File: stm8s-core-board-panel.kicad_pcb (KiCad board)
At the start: 2 copper layers, 95.5 x 95.5 mm, 336 parts, among them IC1 STM8S003F3P, P1 CONN_01X06, P2 USB_OTG, P3 CONN_01X09, P4 CONN_01X09, P5 CONN_01X02, SW1 SW_PUSH, U1 AS1117-5.0, Y1 16MHz

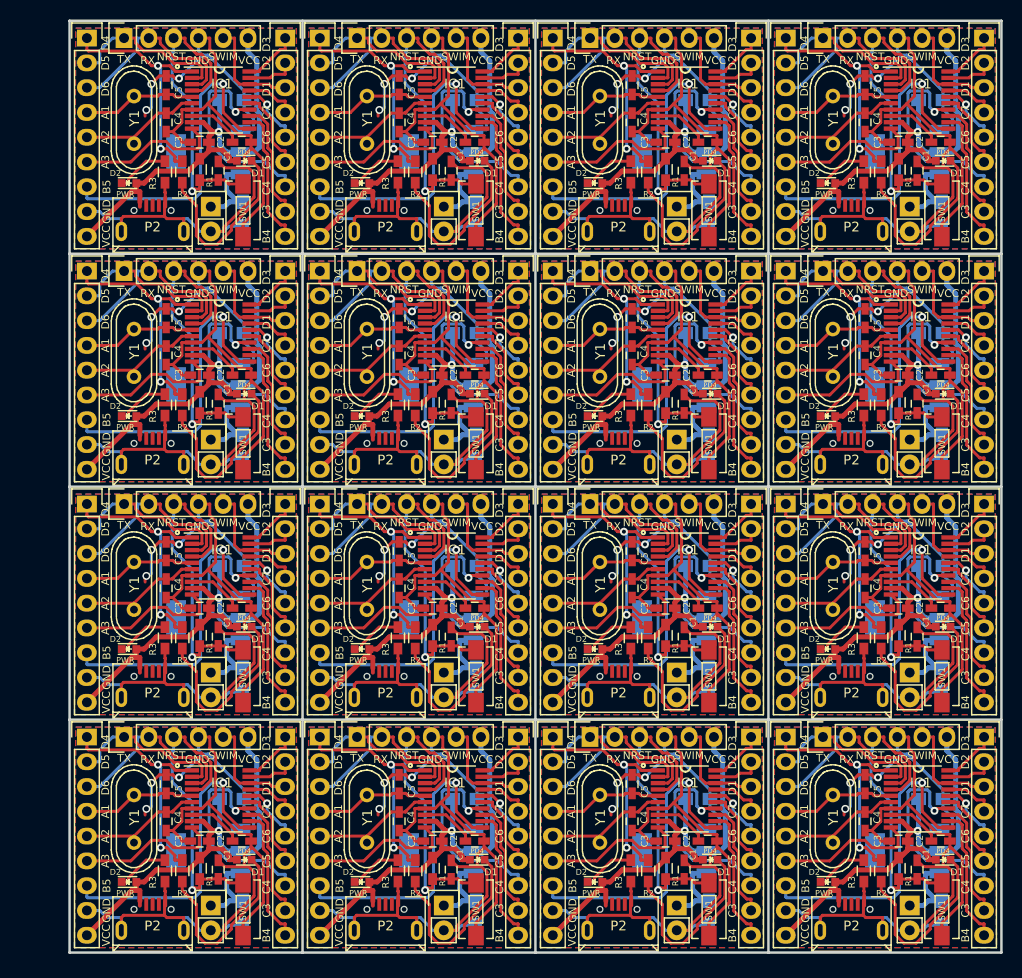
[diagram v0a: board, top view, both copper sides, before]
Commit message: forgot commit for long time. don't know what changed
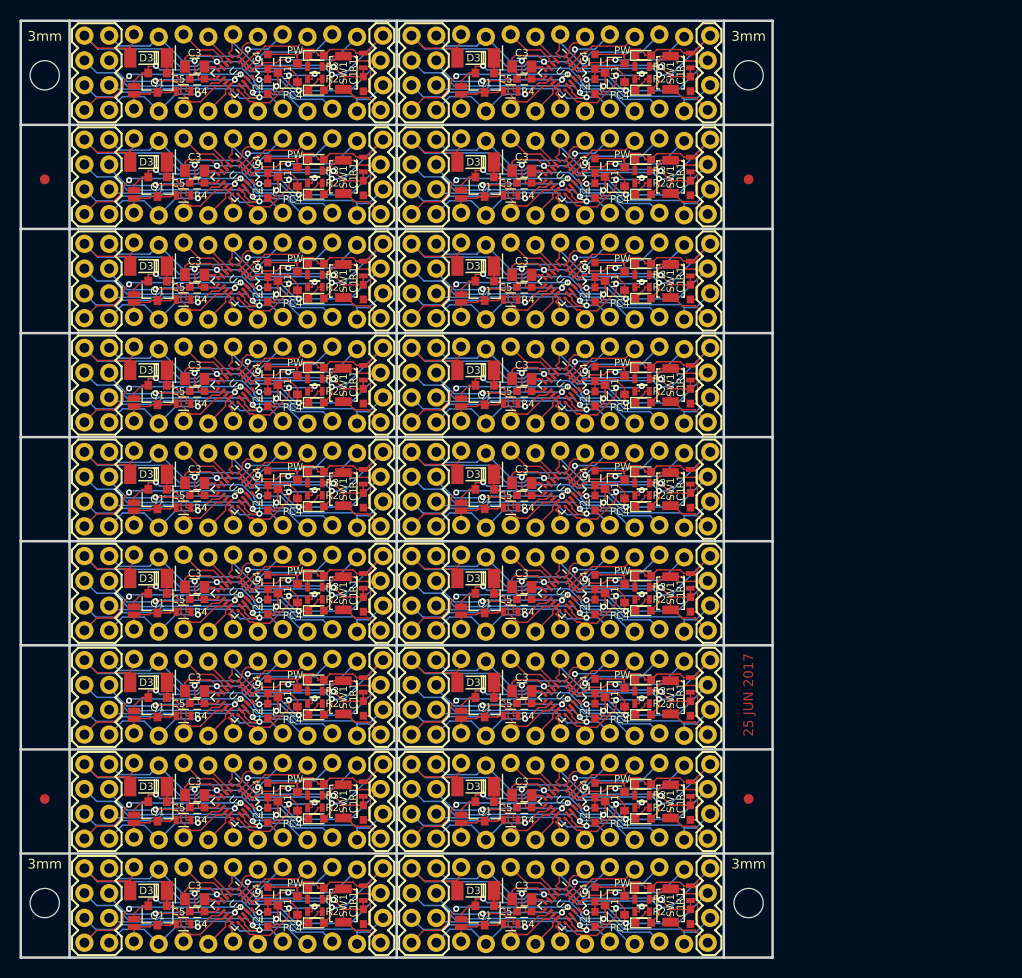
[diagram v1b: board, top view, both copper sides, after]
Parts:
- removed the C1 at (99.6, 99.7)
- removed the C1 at (51.8, 75.8)
- removed the C1 at (51.8, 51.9)
- removed the C1 at (51.8, 28.1)
- removed the C1 at (27.9, 99.7)
- removed the C1 at (27.9, 75.8)
- removed the C1 at (27.9, 51.9)
- removed the C1 at (27.9, 28.1)
- removed the C1 at (99.6, 75.8)
- removed the C1 at (99.6, 51.9)
- removed the C1 at (99.6, 28.1)
- removed the C1 at (75.7, 99.7)
- removed the C1 at (75.7, 75.8)
- removed the C1 at (75.7, 51.9)
- removed the C1 at (75.7, 28.1)
- removed the C1 at (51.8, 99.7)
- removed the C2 at (102.0, 96.8)
- removed the C2 at (54.2, 72.9)
- removed the C2 at (54.2, 49.0)
- removed the C2 at (54.2, 25.1)
- removed the C2 at (30.4, 96.8)
- removed the C2 at (30.4, 72.9)
- removed the C2 at (30.4, 49.0)
- removed the C2 at (30.4, 25.1)
- removed the C2 at (102.0, 72.9)
- removed the C2 at (102.0, 49.0)
- removed the C2 at (102.0, 25.1)
- removed the C2 at (78.1, 96.8)
- removed the C2 at (78.1, 72.9)
- removed the C2 at (78.1, 49.0)
- removed the C2 at (78.1, 25.1)
- removed the C2 at (54.2, 96.8)
- removed the C3 at (97.7, 96.8)
- removed the C3 at (49.9, 72.9)
- removed the C3 at (49.9, 49.0)
- removed the C3 at (49.9, 25.1)
- removed the C3 at (26.0, 96.8)
- removed the C3 at (26.0, 72.9)
- removed the C3 at (26.0, 49.0)
- removed the C3 at (26.0, 25.1)
- removed the C3 at (97.7, 72.9)
- removed the C3 at (97.7, 49.0)
- removed the C3 at (97.7, 25.1)
- removed the C3 at (73.8, 96.8)
- removed the C3 at (73.8, 72.9)
- removed the C3 at (73.8, 49.0)
- removed the C3 at (73.8, 25.1)
- removed the C3 at (49.9, 96.8)
- removed the C4 at (94.2, 94.7)
- removed the C4 at (46.5, 70.9)
- removed the C4 at (46.5, 47.0)
- removed the C4 at (46.5, 23.1)
- removed the C4 at (22.6, 94.7)
- removed the C4 at (22.6, 70.9)
- removed the C4 at (22.6, 47.0)
- removed the C4 at (22.6, 23.1)
- removed the C4 at (94.2, 70.9)
- removed the C4 at (94.2, 47.0)
- removed the C4 at (94.2, 23.1)
- removed the C4 at (70.4, 94.7)
- removed the C4 at (70.4, 70.9)
- removed the C4 at (70.4, 47.0)
- removed the C4 at (70.4, 23.1)
- removed the C4 at (46.5, 94.7)
- removed the C5 at (94.2, 90.9)
- removed the C5 at (46.5, 67.1)
- removed the C5 at (46.5, 43.2)
- removed the C5 at (46.5, 19.3)
- removed the C5 at (22.6, 90.9)
- removed the C5 at (22.6, 67.1)
- removed the C5 at (22.6, 43.2)
- removed the C5 at (22.6, 19.3)
- removed the C5 at (94.2, 67.1)
- removed the C5 at (94.2, 43.2)
- removed the C5 at (94.2, 19.3)
- removed the C5 at (70.4, 90.9)
- removed the C5 at (70.4, 67.1)
- removed the C5 at (70.4, 43.2)
- removed the C5 at (70.4, 19.3)
- removed the C5 at (46.5, 90.9)
- removed C6 (x16), C7 (x16): 10uF, Capacitors_SMD:C_0805_HandSoldering
- removed the D1 at (102.2, 98.7)
- removed the D1 at (54.5, 74.8)
- removed the D1 at (54.5, 50.9)
- removed the D1 at (54.5, 27.1)
- removed the D1 at (30.6, 98.7)
- removed the D1 at (30.6, 74.8)
- removed the D1 at (30.6, 50.9)
- removed the D1 at (30.6, 27.1)
- removed the D1 at (102.2, 74.8)
- removed the D1 at (102.2, 50.9)
- removed the D1 at (102.2, 27.1)
- removed the D1 at (78.4, 98.7)
- removed the D1 at (78.4, 74.8)
- removed the D1 at (78.4, 50.9)
- removed the D1 at (78.4, 27.1)
- removed the D1 at (54.5, 98.7)
- removed the D2 at (90.4, 101.0)
- removed the D2 at (42.7, 77.1)
- removed the D2 at (42.7, 53.2)
- removed the D2 at (42.7, 29.3)
- removed the D2 at (18.8, 101.0)
- removed the D2 at (18.8, 77.1)
- removed the D2 at (18.8, 53.2)
- removed the D2 at (18.8, 29.3)
- removed the D2 at (90.4, 77.1)
- removed the D2 at (90.4, 53.2)
- removed the D2 at (90.4, 29.3)
- removed the D2 at (66.5, 101.0)
- removed the D2 at (66.5, 77.1)
- removed the D2 at (66.5, 53.2)
- removed the D2 at (66.5, 29.3)
- removed the D2 at (42.7, 101.0)
- removed IC1 (x16): STM8S003F3P, Housings_SSOP:TSSOP-20_4.4x6.5mm_Pitch0.65mm
- removed P1 (x16): CONN_01X06, Pin_Headers:Pin_Header_Straight_1x06
- removed P2 (x16): USB_OTG, USB_Micro-B_MK5P
- removed P3 (x16), P4 (x16): CONN_01X09, Pin_Headers:Pin_Header_Straight_1x09
- removed P5 (x16): CONN_01X02, Pin_Headers:Pin_Header_Straight_1x02
- removed the R1 at (97.7, 99.6)
- removed the R1 at (49.9, 75.7)
- removed the R1 at (49.9, 51.8)
- removed the R1 at (49.9, 27.9)
- removed the R1 at (26.0, 99.6)
- removed the R1 at (26.0, 75.7)
- removed the R1 at (26.0, 51.8)
- removed the R1 at (26.0, 27.9)
- removed the R1 at (97.7, 75.7)
- removed the R1 at (97.7, 51.8)
- removed the R1 at (97.7, 27.9)
- removed the R1 at (73.8, 99.6)
- removed the R1 at (73.8, 75.7)
- removed the R1 at (73.8, 51.8)
- removed the R1 at (73.8, 27.9)
- removed the R1 at (49.9, 99.6)
- removed the R2 at (95.9, 99.8)
- removed the R2 at (48.1, 75.9)
- removed the R2 at (48.1, 52.1)
- removed the R2 at (48.1, 28.2)
- removed the R2 at (24.3, 99.8)
- removed the R2 at (24.3, 75.9)
- removed the R2 at (24.3, 52.1)
- removed the R2 at (24.3, 28.2)
- removed the R2 at (95.9, 75.9)
- removed the R2 at (95.9, 52.1)
- removed the R2 at (95.9, 28.2)
- removed the R2 at (72.0, 99.8)
- removed the R2 at (72.0, 75.9)
- removed the R2 at (72.0, 52.1)
- removed the R2 at (72.0, 28.2)
- removed the R2 at (48.1, 99.8)
- removed the R3 at (94.1, 99.8)
- removed the R3 at (46.4, 75.9)
- removed the R3 at (46.4, 52.1)
- removed the R3 at (46.4, 28.2)
- removed the R3 at (22.5, 99.8)
- removed the R3 at (22.5, 75.9)
- removed the R3 at (22.5, 52.1)
- removed the R3 at (22.5, 28.2)
- removed the R3 at (94.1, 75.9)
- removed the R3 at (94.1, 52.1)
- removed the R3 at (94.1, 28.2)
- removed the R3 at (70.2, 99.8)
- removed the R3 at (70.2, 75.9)
- removed the R3 at (70.2, 52.1)
- removed the R3 at (70.2, 28.2)
- removed the R3 at (46.4, 99.8)
- removed the SW1 at (102.1, 103.8)
- removed the SW1 at (54.4, 79.9)
- removed the SW1 at (54.4, 56.0)
- removed the SW1 at (54.4, 32.1)
- removed the SW1 at (30.5, 103.8)
- removed the SW1 at (30.5, 79.9)
- removed the SW1 at (30.5, 56.0)
- removed the SW1 at (30.5, 32.1)
- removed the SW1 at (102.1, 79.9)
- removed the SW1 at (102.1, 56.0)
- removed the SW1 at (102.1, 32.1)
- removed the SW1 at (78.2, 103.8)
- removed the SW1 at (78.2, 79.9)
- removed the SW1 at (78.2, 56.0)
- removed the SW1 at (78.2, 32.1)
- removed the SW1 at (54.4, 103.8)
- removed the U1 at (98.6, 97.8)
- removed the U1 at (50.8, 73.9)
- removed the U1 at (50.8, 50.0)
- removed the U1 at (50.8, 26.2)
- removed the U1 at (26.9, 97.8)
- removed the U1 at (26.9, 73.9)
- removed the U1 at (26.9, 50.0)
- removed the U1 at (26.9, 26.2)
- removed the U1 at (98.6, 73.9)
- removed the U1 at (98.6, 50.0)
- removed the U1 at (98.6, 26.2)
- removed the U1 at (74.7, 97.8)
- removed the U1 at (74.7, 73.9)
- removed the U1 at (74.7, 50.0)
- removed the U1 at (74.7, 26.2)
- removed the U1 at (50.8, 97.8)
- removed Y1 (x16): 16MHz, Crystals:Crystal_HC49-U_Vertical
- added 3mm: MountingHole_3mm, Mounting_Holes:MountingHole_3mm, F.Cu at (10.2, 103.1)
- added 3mm: MountingHole_3mm, Mounting_Holes:MountingHole_3mm, F.Cu at (82.3, 103.1)
- added 3mm: MountingHole_3mm, Mounting_Holes:MountingHole_3mm, F.Cu at (10.2, 18.3)
- added 3mm: MountingHole_3mm, Mounting_Holes:MountingHole_3mm, F.Cu at (82.3, 18.3)
- added C1: 0.1uF, Capacitors_SMD:C_0603, F.Cu at (76.3, 104.5)
- added C1: 0.1uF, Capacitors_SMD:C_0603, F.Cu at (42.8, 104.5)
- added C1: 0.1uF, Capacitors_SMD:C_0603, F.Cu at (42.8, 93.9)
- added C1: 0.1uF, Capacitors_SMD:C_0603, F.Cu at (42.8, 83.2)
- added C1: 0.1uF, Capacitors_SMD:C_0603, F.Cu at (42.8, 72.5)
- added C1: 0.1uF, Capacitors_SMD:C_0603, F.Cu at (42.8, 61.8)
- added C1: 0.1uF, Capacitors_SMD:C_0603, F.Cu at (42.8, 51.2)
- added C1: 0.1uF, Capacitors_SMD:C_0603, F.Cu at (42.8, 40.5)
- added C1: 0.1uF, Capacitors_SMD:C_0603, F.Cu at (42.8, 29.8)
- added C1: 0.1uF, Capacitors_SMD:C_0603, F.Cu at (42.8, 19.2)
- added C1: 0.1uF, Capacitors_SMD:C_0603, F.Cu at (76.3, 93.9)
- added C1: 0.1uF, Capacitors_SMD:C_0603, F.Cu at (76.3, 83.2)
- added C1: 0.1uF, Capacitors_SMD:C_0603, F.Cu at (76.3, 72.5)
- added C1: 0.1uF, Capacitors_SMD:C_0603, F.Cu at (76.3, 61.8)
- added C1: 0.1uF, Capacitors_SMD:C_0603, F.Cu at (76.3, 51.2)
- added C1: 0.1uF, Capacitors_SMD:C_0603, F.Cu at (76.3, 40.5)
- added C1: 0.1uF, Capacitors_SMD:C_0603, F.Cu at (76.3, 29.8)
- added C1: 0.1uF, Capacitors_SMD:C_0603, F.Cu at (76.3, 19.2)
- added C2: 1uF, Capacitors_SMD:C_0603, F.Cu at (66.5, 104.8)
- added C2: 1uF, Capacitors_SMD:C_0603, F.Cu at (33.0, 104.8)
- added C2: 1uF, Capacitors_SMD:C_0603, F.Cu at (33.0, 94.1)
- added C2: 1uF, Capacitors_SMD:C_0603, F.Cu at (33.0, 83.4)
- added C2: 1uF, Capacitors_SMD:C_0603, F.Cu at (33.0, 72.8)
- added C2: 1uF, Capacitors_SMD:C_0603, F.Cu at (33.0, 62.1)
- added C2: 1uF, Capacitors_SMD:C_0603, F.Cu at (33.0, 51.4)
- added C2: 1uF, Capacitors_SMD:C_0603, F.Cu at (33.0, 40.8)
- added C2: 1uF, Capacitors_SMD:C_0603, F.Cu at (33.0, 30.1)
- added C2: 1uF, Capacitors_SMD:C_0603, F.Cu at (33.0, 19.4)
- added C2: 1uF, Capacitors_SMD:C_0603, F.Cu at (66.5, 94.1)
- added C2: 1uF, Capacitors_SMD:C_0603, F.Cu at (66.5, 83.4)
- added C2: 1uF, Capacitors_SMD:C_0603, F.Cu at (66.5, 72.8)
- added C2: 1uF, Capacitors_SMD:C_0603, F.Cu at (66.5, 62.1)
- added C2: 1uF, Capacitors_SMD:C_0603, F.Cu at (66.5, 51.4)
- added C2: 1uF, Capacitors_SMD:C_0603, F.Cu at (66.5, 40.8)
- added C2: 1uF, Capacitors_SMD:C_0603, F.Cu at (66.5, 30.1)
- added C2: 1uF, Capacitors_SMD:C_0603, F.Cu at (66.5, 19.4)
- added C3: 1.0uF, Capacitors_SMD:C_0805, F.Cu at (59.1, 102.7)
- added C3: 1.0uF, Capacitors_SMD:C_0805, F.Cu at (25.5, 102.7)
- added C3: 1.0uF, Capacitors_SMD:C_0805, F.Cu at (25.5, 92.1)
- added C3: 1.0uF, Capacitors_SMD:C_0805, F.Cu at (25.5, 81.4)
- added C3: 1.0uF, Capacitors_SMD:C_0805, F.Cu at (25.5, 70.7)
- added C3: 1.0uF, Capacitors_SMD:C_0805, F.Cu at (25.5, 60.1)
- added C3: 1.0uF, Capacitors_SMD:C_0805, F.Cu at (25.5, 49.4)
- added C3: 1.0uF, Capacitors_SMD:C_0805, F.Cu at (25.5, 38.7)
- added C3: 1.0uF, Capacitors_SMD:C_0805, F.Cu at (25.5, 28.1)
- added C3: 1.0uF, Capacitors_SMD:C_0805, F.Cu at (25.5, 17.4)
- added C3: 1.0uF, Capacitors_SMD:C_0805, F.Cu at (59.1, 92.1)
- added C3: 1.0uF, Capacitors_SMD:C_0805, F.Cu at (59.1, 81.4)
- added C3: 1.0uF, Capacitors_SMD:C_0805, F.Cu at (59.1, 70.7)
- added C3: 1.0uF, Capacitors_SMD:C_0805, F.Cu at (59.1, 60.1)
- added C3: 1.0uF, Capacitors_SMD:C_0805, F.Cu at (59.1, 49.4)
- added C3: 1.0uF, Capacitors_SMD:C_0805, F.Cu at (59.1, 38.7)
- added C3: 1.0uF, Capacitors_SMD:C_0805, F.Cu at (59.1, 28.1)
- added C3: 1.0uF, Capacitors_SMD:C_0805, F.Cu at (59.1, 17.4)
- added C4: 1uF, Capacitors_SMD:C_0603, F.Cu at (66.5, 102.2)
- added C4: 1uF, Capacitors_SMD:C_0603, F.Cu at (33.0, 102.2)
- added C4: 1uF, Capacitors_SMD:C_0603, F.Cu at (33.0, 91.6)
- added C4: 1uF, Capacitors_SMD:C_0603, F.Cu at (33.0, 80.9)
- added C4: 1uF, Capacitors_SMD:C_0603, F.Cu at (33.0, 70.2)
- added C4: 1uF, Capacitors_SMD:C_0603, F.Cu at (33.0, 59.6)
- added C4: 1uF, Capacitors_SMD:C_0603, F.Cu at (33.0, 48.9)
- added C4: 1uF, Capacitors_SMD:C_0603, F.Cu at (33.0, 38.2)
- added C4: 1uF, Capacitors_SMD:C_0603, F.Cu at (33.0, 27.6)
- added C4: 1uF, Capacitors_SMD:C_0603, F.Cu at (33.0, 16.9)
- added C4: 1uF, Capacitors_SMD:C_0603, F.Cu at (66.5, 91.6)
- added C4: 1uF, Capacitors_SMD:C_0603, F.Cu at (66.5, 80.9)
- added C4: 1uF, Capacitors_SMD:C_0603, F.Cu at (66.5, 70.2)
- added C4: 1uF, Capacitors_SMD:C_0603, F.Cu at (66.5, 59.6)
- added C4: 1uF, Capacitors_SMD:C_0603, F.Cu at (66.5, 48.9)
- added C4: 1uF, Capacitors_SMD:C_0603, F.Cu at (66.5, 38.2)
- added C4: 1uF, Capacitors_SMD:C_0603, F.Cu at (66.5, 27.6)
- added C4: 1uF, Capacitors_SMD:C_0603, F.Cu at (66.5, 16.9)
- added C5: 0.1uF, Capacitors_SMD:C_0603, F.Cu at (59.3, 104.0)
- added C5: 0.1uF, Capacitors_SMD:C_0603, F.Cu at (25.8, 104.0)
- added C5: 0.1uF, Capacitors_SMD:C_0603, F.Cu at (25.8, 93.3)
- added C5: 0.1uF, Capacitors_SMD:C_0603, F.Cu at (25.8, 82.7)
- added C5: 0.1uF, Capacitors_SMD:C_0603, F.Cu at (25.8, 72.0)
- added C5: 0.1uF, Capacitors_SMD:C_0603, F.Cu at (25.8, 61.3)
- added C5: 0.1uF, Capacitors_SMD:C_0603, F.Cu at (25.8, 50.7)
- added C5: 0.1uF, Capacitors_SMD:C_0603, F.Cu at (25.8, 40.0)
- added C5: 0.1uF, Capacitors_SMD:C_0603, F.Cu at (25.8, 29.3)
- added C5: 0.1uF, Capacitors_SMD:C_0603, F.Cu at (25.8, 18.7)
- added C5: 0.1uF, Capacitors_SMD:C_0603, F.Cu at (59.3, 93.3)
- added C5: 0.1uF, Capacitors_SMD:C_0603, F.Cu at (59.3, 82.7)
- added C5: 0.1uF, Capacitors_SMD:C_0603, F.Cu at (59.3, 72.0)
- added C5: 0.1uF, Capacitors_SMD:C_0603, F.Cu at (59.3, 61.3)
- added C5: 0.1uF, Capacitors_SMD:C_0603, F.Cu at (59.3, 50.7)
- added C5: 0.1uF, Capacitors_SMD:C_0603, F.Cu at (59.3, 40.0)
- added C5: 0.1uF, Capacitors_SMD:C_0603, F.Cu at (59.3, 29.3)
- added C5: 0.1uF, Capacitors_SMD:C_0603, F.Cu at (59.3, 18.7)
- added D1: BLUE, LEDs:LED_0603, F.Cu at (71.5, 105.2)
- added D1: BLUE, LEDs:LED_0603, F.Cu at (38.0, 105.2)
- added D1: BLUE, LEDs:LED_0603, F.Cu at (38.0, 94.5)
- added D1: BLUE, LEDs:LED_0603, F.Cu at (38.0, 83.8)
- added D1: BLUE, LEDs:LED_0603, F.Cu at (38.0, 73.2)
- added D1: BLUE, LEDs:LED_0603, F.Cu at (38.0, 62.5)
- added D1: BLUE, LEDs:LED_0603, F.Cu at (38.0, 51.8)
- added D1: BLUE, LEDs:LED_0603, F.Cu at (38.0, 41.1)
- added D1: BLUE, LEDs:LED_0603, F.Cu at (38.0, 30.5)
- added D1: BLUE, LEDs:LED_0603, F.Cu at (38.0, 19.8)
- added D1: BLUE, LEDs:LED_0603, F.Cu at (71.5, 94.5)
- added D1: BLUE, LEDs:LED_0603, F.Cu at (71.5, 83.8)
- added D1: BLUE, LEDs:LED_0603, F.Cu at (71.5, 73.2)
- added D1: BLUE, LEDs:LED_0603, F.Cu at (71.5, 62.5)
- added D1: BLUE, LEDs:LED_0603, F.Cu at (71.5, 51.8)
- added D1: BLUE, LEDs:LED_0603, F.Cu at (71.5, 41.1)
- added D1: BLUE, LEDs:LED_0603, F.Cu at (71.5, 30.5)
- added D1: BLUE, LEDs:LED_0603, F.Cu at (71.5, 19.8)
- added D2: RED, LEDs:LED_0603, F.Cu at (71.5, 101.6)
- added D2: RED, LEDs:LED_0603, F.Cu at (38.0, 101.6)
- added D2: RED, LEDs:LED_0603, F.Cu at (38.0, 90.9)
- added D2: RED, LEDs:LED_0603, F.Cu at (38.0, 80.3)
- added D2: RED, LEDs:LED_0603, F.Cu at (38.0, 69.6)
- added D2: RED, LEDs:LED_0603, F.Cu at (38.0, 58.9)
- added D2: RED, LEDs:LED_0603, F.Cu at (38.0, 48.3)
- added D2: RED, LEDs:LED_0603, F.Cu at (38.0, 37.6)
- added D2: RED, LEDs:LED_0603, F.Cu at (38.0, 26.9)
- added D2: RED, LEDs:LED_0603, F.Cu at (38.0, 16.3)
- added D2: RED, LEDs:LED_0603, F.Cu at (71.5, 90.9)
- added D2: RED, LEDs:LED_0603, F.Cu at (71.5, 80.3)
- added D2: RED, LEDs:LED_0603, F.Cu at (71.5, 69.6)
- added D2: RED, LEDs:LED_0603, F.Cu at (71.5, 58.9)
- added D2: RED, LEDs:LED_0603, F.Cu at (71.5, 48.3)
- added D2: RED, LEDs:LED_0603, F.Cu at (71.5, 37.6)
- added D2: RED, LEDs:LED_0603, F.Cu at (71.5, 26.9)
- added D2: RED, LEDs:LED_0603, F.Cu at (71.5, 16.3)
- added D3: 5.6V, MyOwn:SOD-80, F.Cu at (54.3, 101.9)
- added D3: 5.6V, MyOwn:SOD-80, F.Cu at (20.8, 101.9)
- added D3: 5.6V, MyOwn:SOD-80, F.Cu at (20.8, 91.2)
- added D3: 5.6V, MyOwn:SOD-80, F.Cu at (20.8, 80.5)
- added D3: 5.6V, MyOwn:SOD-80, F.Cu at (20.8, 69.8)
- added D3: 5.6V, MyOwn:SOD-80, F.Cu at (20.8, 59.2)
- added D3: 5.6V, MyOwn:SOD-80, F.Cu at (20.8, 48.5)
- added D3: 5.6V, MyOwn:SOD-80, F.Cu at (20.8, 37.8)
- added D3: 5.6V, MyOwn:SOD-80, F.Cu at (20.8, 27.2)
- added D3: 5.6V, MyOwn:SOD-80, F.Cu at (20.8, 16.5)
- added D3: 5.6V, MyOwn:SOD-80, F.Cu at (54.3, 91.2)
- added D3: 5.6V, MyOwn:SOD-80, F.Cu at (54.3, 80.5)
- added D3: 5.6V, MyOwn:SOD-80, F.Cu at (54.3, 69.8)
- added D3: 5.6V, MyOwn:SOD-80, F.Cu at (54.3, 59.2)
- added D3: 5.6V, MyOwn:SOD-80, F.Cu at (54.3, 48.5)
- added D3: 5.6V, MyOwn:SOD-80, F.Cu at (54.3, 37.8)
- added D3: 5.6V, MyOwn:SOD-80, F.Cu at (54.3, 27.2)
- added D3: 5.6V, MyOwn:SOD-80, F.Cu at (54.3, 16.5)
- added J1: CONN_01X04, SparkFun-Connectors:1X04_LOCK, F.Cu at (78.2, 107.2)
- added J1: CONN_01X04, SparkFun-Connectors:1X04_LOCK, F.Cu at (44.7, 107.2)
- added J1: CONN_01X04, SparkFun-Connectors:1X04_LOCK, F.Cu at (44.7, 96.5)
- added J1: CONN_01X04, SparkFun-Connectors:1X04_LOCK, F.Cu at (44.7, 85.9)
- added J1: CONN_01X04, SparkFun-Connectors:1X04_LOCK, F.Cu at (44.7, 75.2)
- added J1: CONN_01X04, SparkFun-Connectors:1X04_LOCK, F.Cu at (44.7, 64.5)
- added J1: CONN_01X04, SparkFun-Connectors:1X04_LOCK, F.Cu at (44.7, 53.8)
- added J1: CONN_01X04, SparkFun-Connectors:1X04_LOCK, F.Cu at (44.7, 43.2)
- added J1: CONN_01X04, SparkFun-Connectors:1X04_LOCK, F.Cu at (44.7, 32.5)
- added J1: CONN_01X04, SparkFun-Connectors:1X04_LOCK, F.Cu at (44.7, 21.8)
- added J1: CONN_01X04, SparkFun-Connectors:1X04_LOCK, F.Cu at (78.2, 96.5)
- added J1: CONN_01X04, SparkFun-Connectors:1X04_LOCK, F.Cu at (78.2, 85.9)
- added J1: CONN_01X04, SparkFun-Connectors:1X04_LOCK, F.Cu at (78.2, 75.2)
- added J1: CONN_01X04, SparkFun-Connectors:1X04_LOCK, F.Cu at (78.2, 64.5)
- added J1: CONN_01X04, SparkFun-Connectors:1X04_LOCK, F.Cu at (78.2, 53.8)
- added J1: CONN_01X04, SparkFun-Connectors:1X04_LOCK, F.Cu at (78.2, 43.2)
- added J1: CONN_01X04, SparkFun-Connectors:1X04_LOCK, F.Cu at (78.2, 32.5)
- added J1: CONN_01X04, SparkFun-Connectors:1X04_LOCK, F.Cu at (78.2, 21.8)
- added J2: CONN_02X04, SparkFun-Connectors:2X4, F.Cu at (49.0, 103.4)
- added J2: CONN_02X04, SparkFun-Connectors:2X4, F.Cu at (15.5, 103.4)
- added J2: CONN_02X04, SparkFun-Connectors:2X4, F.Cu at (15.5, 92.7)
- added J2: CONN_02X04, SparkFun-Connectors:2X4, F.Cu at (15.5, 82.0)
- added J2: CONN_02X04, SparkFun-Connectors:2X4, F.Cu at (15.5, 71.4)
- added J2: CONN_02X04, SparkFun-Connectors:2X4, F.Cu at (15.5, 60.7)
- added J2: CONN_02X04, SparkFun-Connectors:2X4, F.Cu at (15.5, 50.0)
- added J2: CONN_02X04, SparkFun-Connectors:2X4, F.Cu at (15.5, 39.4)
- added J2: CONN_02X04, SparkFun-Connectors:2X4, F.Cu at (15.5, 28.7)
- added J2: CONN_02X04, SparkFun-Connectors:2X4, F.Cu at (15.5, 18.0)
- added J2: CONN_02X04, SparkFun-Connectors:2X4, F.Cu at (49.0, 92.7)
- added J2: CONN_02X04, SparkFun-Connectors:2X4, F.Cu at (49.0, 82.0)
- added J2: CONN_02X04, SparkFun-Connectors:2X4, F.Cu at (49.0, 71.4)
- added J2: CONN_02X04, SparkFun-Connectors:2X4, F.Cu at (49.0, 60.7)
- added J2: CONN_02X04, SparkFun-Connectors:2X4, F.Cu at (49.0, 50.0)
- added J2: CONN_02X04, SparkFun-Connectors:2X4, F.Cu at (49.0, 39.4)
- added J2: CONN_02X04, SparkFun-Connectors:2X4, F.Cu at (49.0, 28.7)
- added J2: CONN_02X04, SparkFun-Connectors:2X4, F.Cu at (49.0, 18.0)
- added J3: CONN_01X10, SparkFun-Connectors:1X10_LOCK_NS, F.Cu at (52.8, 107.2)
- added J3: CONN_01X10, SparkFun-Connectors:1X10_LOCK_NS, F.Cu at (19.3, 107.2)
- added J3: CONN_01X10, SparkFun-Connectors:1X10_LOCK_NS, F.Cu at (19.3, 96.5)
- added J3: CONN_01X10, SparkFun-Connectors:1X10_LOCK_NS, F.Cu at (19.3, 85.9)
- added J3: CONN_01X10, SparkFun-Connectors:1X10_LOCK_NS, F.Cu at (19.3, 75.2)
- added J3: CONN_01X10, SparkFun-Connectors:1X10_LOCK_NS, F.Cu at (19.3, 64.5)
- added J3: CONN_01X10, SparkFun-Connectors:1X10_LOCK_NS, F.Cu at (19.3, 53.8)
- added J3: CONN_01X10, SparkFun-Connectors:1X10_LOCK_NS, F.Cu at (19.3, 43.2)
- added J3: CONN_01X10, SparkFun-Connectors:1X10_LOCK_NS, F.Cu at (19.3, 32.5)
- added J3: CONN_01X10, SparkFun-Connectors:1X10_LOCK_NS, F.Cu at (19.3, 21.8)
- added J3: CONN_01X10, SparkFun-Connectors:1X10_LOCK_NS, F.Cu at (52.8, 96.5)
- added J3: CONN_01X10, SparkFun-Connectors:1X10_LOCK_NS, F.Cu at (52.8, 85.9)
- added J3: CONN_01X10, SparkFun-Connectors:1X10_LOCK_NS, F.Cu at (52.8, 75.2)
- added J3: CONN_01X10, SparkFun-Connectors:1X10_LOCK_NS, F.Cu at (52.8, 64.5)
- added J3: CONN_01X10, SparkFun-Connectors:1X10_LOCK_NS, F.Cu at (52.8, 53.8)
- added J3: CONN_01X10, SparkFun-Connectors:1X10_LOCK_NS, F.Cu at (52.8, 43.2)
- added J3: CONN_01X10, SparkFun-Connectors:1X10_LOCK_NS, F.Cu at (52.8, 32.5)
- added J3: CONN_01X10, SparkFun-Connectors:1X10_LOCK_NS, F.Cu at (52.8, 21.8)
- added J4: CONN_01X10, SparkFun-Connectors:1X10_LOCK_NS, F.Cu at (52.8, 99.6)
- added J4: CONN_01X10, SparkFun-Connectors:1X10_LOCK_NS, F.Cu at (19.3, 99.6)
- added J4: CONN_01X10, SparkFun-Connectors:1X10_LOCK_NS, F.Cu at (19.3, 88.9)
- added J4: CONN_01X10, SparkFun-Connectors:1X10_LOCK_NS, F.Cu at (19.3, 78.2)
- added J4: CONN_01X10, SparkFun-Connectors:1X10_LOCK_NS, F.Cu at (19.3, 67.6)
- added J4: CONN_01X10, SparkFun-Connectors:1X10_LOCK_NS, F.Cu at (19.3, 56.9)
- added J4: CONN_01X10, SparkFun-Connectors:1X10_LOCK_NS, F.Cu at (19.3, 46.2)
- added J4: CONN_01X10, SparkFun-Connectors:1X10_LOCK_NS, F.Cu at (19.3, 35.6)
- added J4: CONN_01X10, SparkFun-Connectors:1X10_LOCK_NS, F.Cu at (19.3, 24.9)
- added J4: CONN_01X10, SparkFun-Connectors:1X10_LOCK_NS, F.Cu at (19.3, 14.2)
- added J4: CONN_01X10, SparkFun-Connectors:1X10_LOCK_NS, F.Cu at (52.8, 88.9)
- added J4: CONN_01X10, SparkFun-Connectors:1X10_LOCK_NS, F.Cu at (52.8, 78.2)
- added J4: CONN_01X10, SparkFun-Connectors:1X10_LOCK_NS, F.Cu at (52.8, 67.6)
- added J4: CONN_01X10, SparkFun-Connectors:1X10_LOCK_NS, F.Cu at (52.8, 56.9)
- added J4: CONN_01X10, SparkFun-Connectors:1X10_LOCK_NS, F.Cu at (52.8, 46.2)
- added J4: CONN_01X10, SparkFun-Connectors:1X10_LOCK_NS, F.Cu at (52.8, 35.6)
- added J4: CONN_01X10, SparkFun-Connectors:1X10_LOCK_NS, F.Cu at (52.8, 24.9)
- added J4: CONN_01X10, SparkFun-Connectors:1X10_LOCK_NS, F.Cu at (52.8, 14.2)
- added JP2: 12V-30V input, SparkFun-Jumpers:SMT-JUMPER_2_NO_NO-SILK, F.Cu at (52.8, 105.2)
- added JP2: 12V-30V input, SparkFun-Jumpers:SMT-JUMPER_2_NO_NO-SILK, F.Cu at (19.3, 105.2)
- added JP2: 12V-30V input, SparkFun-Jumpers:SMT-JUMPER_2_NO_NO-SILK, F.Cu at (19.3, 94.5)
- added JP2: 12V-30V input, SparkFun-Jumpers:SMT-JUMPER_2_NO_NO-SILK, F.Cu at (19.3, 83.8)
- added JP2: 12V-30V input, SparkFun-Jumpers:SMT-JUMPER_2_NO_NO-SILK, F.Cu at (19.3, 73.2)
- added JP2: 12V-30V input, SparkFun-Jumpers:SMT-JUMPER_2_NO_NO-SILK, F.Cu at (19.3, 62.5)
- added JP2: 12V-30V input, SparkFun-Jumpers:SMT-JUMPER_2_NO_NO-SILK, F.Cu at (19.3, 51.8)
- added JP2: 12V-30V input, SparkFun-Jumpers:SMT-JUMPER_2_NO_NO-SILK, F.Cu at (19.3, 41.1)
- added JP2: 12V-30V input, SparkFun-Jumpers:SMT-JUMPER_2_NO_NO-SILK, F.Cu at (19.3, 30.5)
- added JP2: 12V-30V input, SparkFun-Jumpers:SMT-JUMPER_2_NO_NO-SILK, F.Cu at (19.3, 19.8)
- added JP2: 12V-30V input, SparkFun-Jumpers:SMT-JUMPER_2_NO_NO-SILK, F.Cu at (52.8, 94.5)
- added JP2: 12V-30V input, SparkFun-Jumpers:SMT-JUMPER_2_NO_NO-SILK, F.Cu at (52.8, 83.8)
- added JP2: 12V-30V input, SparkFun-Jumpers:SMT-JUMPER_2_NO_NO-SILK, F.Cu at (52.8, 73.2)
- added JP2: 12V-30V input, SparkFun-Jumpers:SMT-JUMPER_2_NO_NO-SILK, F.Cu at (52.8, 62.5)
- added JP2: 12V-30V input, SparkFun-Jumpers:SMT-JUMPER_2_NO_NO-SILK, F.Cu at (52.8, 51.8)
- added JP2: 12V-30V input, SparkFun-Jumpers:SMT-JUMPER_2_NO_NO-SILK, F.Cu at (52.8, 41.1)
- added JP2: 12V-30V input, SparkFun-Jumpers:SMT-JUMPER_2_NO_NO-SILK, F.Cu at (52.8, 30.5)
- added JP2: 12V-30V input, SparkFun-Jumpers:SMT-JUMPER_2_NO_NO-SILK, F.Cu at (52.8, 19.8)
- added Q1: BC817-40, TO_SOT_Packages_SMD:SOT-23, F.Cu at (55.2, 104.4)
- added Q1: BC817-40, TO_SOT_Packages_SMD:SOT-23, F.Cu at (21.7, 104.4)
- added Q1: BC817-40, TO_SOT_Packages_SMD:SOT-23, F.Cu at (21.7, 93.7)
- added Q1: BC817-40, TO_SOT_Packages_SMD:SOT-23, F.Cu at (21.7, 83.1)
- added Q1: BC817-40, TO_SOT_Packages_SMD:SOT-23, F.Cu at (21.7, 72.4)
- added Q1: BC817-40, TO_SOT_Packages_SMD:SOT-23, F.Cu at (21.7, 61.7)
- added Q1: BC817-40, TO_SOT_Packages_SMD:SOT-23, F.Cu at (21.7, 51.1)
- added Q1: BC817-40, TO_SOT_Packages_SMD:SOT-23, F.Cu at (21.7, 40.4)
- added Q1: BC817-40, TO_SOT_Packages_SMD:SOT-23, F.Cu at (21.7, 29.7)
- added Q1: BC817-40, TO_SOT_Packages_SMD:SOT-23, F.Cu at (21.7, 19.1)
- added Q1: BC817-40, TO_SOT_Packages_SMD:SOT-23, F.Cu at (55.2, 93.7)
- added Q1: BC817-40, TO_SOT_Packages_SMD:SOT-23, F.Cu at (55.2, 83.1)
- added Q1: BC817-40, TO_SOT_Packages_SMD:SOT-23, F.Cu at (55.2, 72.4)
- added Q1: BC817-40, TO_SOT_Packages_SMD:SOT-23, F.Cu at (55.2, 61.7)
- added Q1: BC817-40, TO_SOT_Packages_SMD:SOT-23, F.Cu at (55.2, 51.1)
- added Q1: BC817-40, TO_SOT_Packages_SMD:SOT-23, F.Cu at (55.2, 40.4)
- added Q1: BC817-40, TO_SOT_Packages_SMD:SOT-23, F.Cu at (55.2, 29.7)
- added Q1: BC817-40, TO_SOT_Packages_SMD:SOT-23, F.Cu at (55.2, 19.1)
- added R1: 100K, Resistors_SMD:R_0603, F.Cu at (76.3, 102.1)
- added R1: 100K, Resistors_SMD:R_0603, F.Cu at (42.8, 102.1)
- added R1: 100K, Resistors_SMD:R_0603, F.Cu at (42.8, 91.4)
- added R1: 100K, Resistors_SMD:R_0603, F.Cu at (42.8, 80.8)
- added R1: 100K, Resistors_SMD:R_0603, F.Cu at (42.8, 70.1)
- added R1: 100K, Resistors_SMD:R_0603, F.Cu at (42.8, 59.4)
- added R1: 100K, Resistors_SMD:R_0603, F.Cu at (42.8, 48.8)
- added R1: 100K, Resistors_SMD:R_0603, F.Cu at (42.8, 38.1)
- added R1: 100K, Resistors_SMD:R_0603, F.Cu at (42.8, 27.4)
- added R1: 100K, Resistors_SMD:R_0603, F.Cu at (42.8, 16.8)
- added R1: 100K, Resistors_SMD:R_0603, F.Cu at (76.3, 91.4)
- added R1: 100K, Resistors_SMD:R_0603, F.Cu at (76.3, 80.8)
- added R1: 100K, Resistors_SMD:R_0603, F.Cu at (76.3, 70.1)
- added R1: 100K, Resistors_SMD:R_0603, F.Cu at (76.3, 59.4)
- added R1: 100K, Resistors_SMD:R_0603, F.Cu at (76.3, 48.8)
- added R1: 100K, Resistors_SMD:R_0603, F.Cu at (76.3, 38.1)
- added R1: 100K, Resistors_SMD:R_0603, F.Cu at (76.3, 27.4)
- added R1: 100K, Resistors_SMD:R_0603, F.Cu at (76.3, 16.8)
- added R2: 1K, Resistors_SMD:R_0603, F.Cu at (71.4, 104.0)
- added R2: 1K, Resistors_SMD:R_0603, F.Cu at (37.8, 104.0)
- added R2: 1K, Resistors_SMD:R_0603, F.Cu at (37.8, 93.3)
- added R2: 1K, Resistors_SMD:R_0603, F.Cu at (37.8, 82.7)
- added R2: 1K, Resistors_SMD:R_0603, F.Cu at (37.8, 72.0)
- added R2: 1K, Resistors_SMD:R_0603, F.Cu at (37.8, 61.3)
- added R2: 1K, Resistors_SMD:R_0603, F.Cu at (37.8, 50.7)
- added R2: 1K, Resistors_SMD:R_0603, F.Cu at (37.8, 40.0)
- added R2: 1K, Resistors_SMD:R_0603, F.Cu at (37.8, 29.3)
- added R2: 1K, Resistors_SMD:R_0603, F.Cu at (37.8, 18.7)
- added R2: 1K, Resistors_SMD:R_0603, F.Cu at (71.4, 93.3)
- added R2: 1K, Resistors_SMD:R_0603, F.Cu at (71.4, 82.7)
- added R2: 1K, Resistors_SMD:R_0603, F.Cu at (71.4, 72.0)
- added R2: 1K, Resistors_SMD:R_0603, F.Cu at (71.4, 61.3)
- added R2: 1K, Resistors_SMD:R_0603, F.Cu at (71.4, 50.7)
- added R2: 1K, Resistors_SMD:R_0603, F.Cu at (71.4, 40.0)
- added R2: 1K, Resistors_SMD:R_0603, F.Cu at (71.4, 29.3)
- added R2: 1K, Resistors_SMD:R_0603, F.Cu at (71.4, 18.7)
- added R3: 1K, Resistors_SMD:R_0603, F.Cu at (71.4, 102.7)
- added R3: 1K, Resistors_SMD:R_0603, F.Cu at (37.8, 102.7)
- added R3: 1K, Resistors_SMD:R_0603, F.Cu at (37.8, 92.1)
- added R3: 1K, Resistors_SMD:R_0603, F.Cu at (37.8, 81.4)
- added R3: 1K, Resistors_SMD:R_0603, F.Cu at (37.8, 70.7)
- added R3: 1K, Resistors_SMD:R_0603, F.Cu at (37.8, 60.1)
- added R3: 1K, Resistors_SMD:R_0603, F.Cu at (37.8, 49.4)
- added R3: 1K, Resistors_SMD:R_0603, F.Cu at (37.8, 38.7)
- added R3: 1K, Resistors_SMD:R_0603, F.Cu at (37.8, 28.1)
- added R3: 1K, Resistors_SMD:R_0603, F.Cu at (37.8, 17.4)
- added R3: 1K, Resistors_SMD:R_0603, F.Cu at (71.4, 92.1)
- added R3: 1K, Resistors_SMD:R_0603, F.Cu at (71.4, 81.4)
- added R3: 1K, Resistors_SMD:R_0603, F.Cu at (71.4, 70.7)
- added R3: 1K, Resistors_SMD:R_0603, F.Cu at (71.4, 60.1)
- added R3: 1K, Resistors_SMD:R_0603, F.Cu at (71.4, 49.4)
- added R3: 1K, Resistors_SMD:R_0603, F.Cu at (71.4, 38.7)
- added R3: 1K, Resistors_SMD:R_0603, F.Cu at (71.4, 28.1)
- added R3: 1K, Resistors_SMD:R_0603, F.Cu at (71.4, 17.4)
- added R4: 1K, Resistors_SMD:R_0603, F.Cu at (57.9, 105.3)
- added R4: 1K, Resistors_SMD:R_0603, F.Cu at (24.4, 105.3)
- added R4: 1K, Resistors_SMD:R_0603, F.Cu at (24.4, 94.6)
- added R4: 1K, Resistors_SMD:R_0603, F.Cu at (24.4, 83.9)
- added R4: 1K, Resistors_SMD:R_0603, F.Cu at (24.4, 73.3)
- added R4: 1K, Resistors_SMD:R_0603, F.Cu at (24.4, 62.6)
- added R4: 1K, Resistors_SMD:R_0603, F.Cu at (24.4, 51.9)
- added R4: 1K, Resistors_SMD:R_0603, F.Cu at (24.4, 41.3)
- added R4: 1K, Resistors_SMD:R_0603, F.Cu at (24.4, 30.6)
- added R4: 1K, Resistors_SMD:R_0603, F.Cu at (24.4, 19.9)
- added R4: 1K, Resistors_SMD:R_0603, F.Cu at (57.9, 94.6)
- added R4: 1K, Resistors_SMD:R_0603, F.Cu at (57.9, 83.9)
- added R4: 1K, Resistors_SMD:R_0603, F.Cu at (57.9, 73.3)
- added R4: 1K, Resistors_SMD:R_0603, F.Cu at (57.9, 62.6)
- added R4: 1K, Resistors_SMD:R_0603, F.Cu at (57.9, 51.9)
- added R4: 1K, Resistors_SMD:R_0603, F.Cu at (57.9, 41.3)
- added R4: 1K, Resistors_SMD:R_0603, F.Cu at (57.9, 30.6)
- added R4: 1K, Resistors_SMD:R_0603, F.Cu at (57.9, 19.9)
- added REF**: Fiducial_1mm_Dia_2.54mm_Outer_CopperTop, Fiducials:Fiducial_1mm_Dia_2.54mm_Outer_CopperTop, F.Cu at (82.3, 92.5)
- added REF**: Fiducial_1mm_Dia_2.54mm_Outer_CopperTop, Fiducials:Fiducial_1mm_Dia_2.54mm_Outer_CopperTop, F.Cu at (10.2, 92.5)
- added REF**: Fiducial_1mm_Dia_2.54mm_Outer_CopperTop, Fiducials:Fiducial_1mm_Dia_2.54mm_Outer_CopperTop, F.Cu at (10.2, 29.0)
- added REF**: Fiducial_1mm_Dia_2.54mm_Outer_CopperTop, Fiducials:Fiducial_1mm_Dia_2.54mm_Outer_CopperTop, F.Cu at (82.3, 29.0)
- added SW1: SW_PUSH, Buttons_Switches_SMD:SW_SPST_B3U-1000P, F.Cu at (74.3, 103.4)
- added SW1: SW_PUSH, Buttons_Switches_SMD:SW_SPST_B3U-1000P, F.Cu at (40.8, 103.4)
- added SW1: SW_PUSH, Buttons_Switches_SMD:SW_SPST_B3U-1000P, F.Cu at (40.8, 92.7)
- added SW1: SW_PUSH, Buttons_Switches_SMD:SW_SPST_B3U-1000P, F.Cu at (40.8, 82.0)
- added SW1: SW_PUSH, Buttons_Switches_SMD:SW_SPST_B3U-1000P, F.Cu at (40.8, 71.4)
- added SW1: SW_PUSH, Buttons_Switches_SMD:SW_SPST_B3U-1000P, F.Cu at (40.8, 60.7)
- added SW1: SW_PUSH, Buttons_Switches_SMD:SW_SPST_B3U-1000P, F.Cu at (40.8, 50.0)
- added SW1: SW_PUSH, Buttons_Switches_SMD:SW_SPST_B3U-1000P, F.Cu at (40.8, 39.4)
- added SW1: SW_PUSH, Buttons_Switches_SMD:SW_SPST_B3U-1000P, F.Cu at (40.8, 28.7)
- added SW1: SW_PUSH, Buttons_Switches_SMD:SW_SPST_B3U-1000P, F.Cu at (40.8, 18.0)
- added SW1: SW_PUSH, Buttons_Switches_SMD:SW_SPST_B3U-1000P, F.Cu at (74.3, 92.7)
- added SW1: SW_PUSH, Buttons_Switches_SMD:SW_SPST_B3U-1000P, F.Cu at (74.3, 82.0)
- added SW1: SW_PUSH, Buttons_Switches_SMD:SW_SPST_B3U-1000P, F.Cu at (74.3, 71.4)
- added SW1: SW_PUSH, Buttons_Switches_SMD:SW_SPST_B3U-1000P, F.Cu at (74.3, 60.7)
- added SW1: SW_PUSH, Buttons_Switches_SMD:SW_SPST_B3U-1000P, F.Cu at (74.3, 50.0)
- added SW1: SW_PUSH, Buttons_Switches_SMD:SW_SPST_B3U-1000P, F.Cu at (74.3, 39.4)
- added SW1: SW_PUSH, Buttons_Switches_SMD:SW_SPST_B3U-1000P, F.Cu at (74.3, 28.7)
- added SW1: SW_PUSH, Buttons_Switches_SMD:SW_SPST_B3U-1000P, F.Cu at (74.3, 18.0)
- added U1: XC6206, TO_SOT_Packages_SMD:SOT-23, F.Cu at (68.6, 103.4)
- added U1: XC6206, TO_SOT_Packages_SMD:SOT-23, F.Cu at (35.1, 103.4)
- added U1: XC6206, TO_SOT_Packages_SMD:SOT-23, F.Cu at (35.1, 92.7)
- added U1: XC6206, TO_SOT_Packages_SMD:SOT-23, F.Cu at (35.1, 82.0)
- added U1: XC6206, TO_SOT_Packages_SMD:SOT-23, F.Cu at (35.1, 71.4)
- added U1: XC6206, TO_SOT_Packages_SMD:SOT-23, F.Cu at (35.1, 60.7)
- added U1: XC6206, TO_SOT_Packages_SMD:SOT-23, F.Cu at (35.1, 50.0)
- added U1: XC6206, TO_SOT_Packages_SMD:SOT-23, F.Cu at (35.1, 39.4)
- added U1: XC6206, TO_SOT_Packages_SMD:SOT-23, F.Cu at (35.1, 28.7)
- added U1: XC6206, TO_SOT_Packages_SMD:SOT-23, F.Cu at (35.1, 18.0)
- added U1: XC6206, TO_SOT_Packages_SMD:SOT-23, F.Cu at (68.6, 92.7)
- added U1: XC6206, TO_SOT_Packages_SMD:SOT-23, F.Cu at (68.6, 82.0)
- added U1: XC6206, TO_SOT_Packages_SMD:SOT-23, F.Cu at (68.6, 71.4)
- added U1: XC6206, TO_SOT_Packages_SMD:SOT-23, F.Cu at (68.6, 60.7)
- added U1: XC6206, TO_SOT_Packages_SMD:SOT-23, F.Cu at (68.6, 50.0)
- added U1: XC6206, TO_SOT_Packages_SMD:SOT-23, F.Cu at (68.6, 39.4)
- added U1: XC6206, TO_SOT_Packages_SMD:SOT-23, F.Cu at (68.6, 28.7)
- added U1: XC6206, TO_SOT_Packages_SMD:SOT-23, F.Cu at (68.6, 18.0)
- added U2: STM8S003F3U, MyOwn:UQFN-16_3x3mm_Pitch0.5mm, F.Cu at (63.2, 103.4)
- added U2: STM8S003F3U, MyOwn:UQFN-16_3x3mm_Pitch0.5mm, F.Cu at (29.7, 103.4)
- added U2: STM8S003F3U, MyOwn:UQFN-16_3x3mm_Pitch0.5mm, F.Cu at (29.7, 92.8)
- added U2: STM8S003F3U, MyOwn:UQFN-16_3x3mm_Pitch0.5mm, F.Cu at (29.7, 82.1)
- added U2: STM8S003F3U, MyOwn:UQFN-16_3x3mm_Pitch0.5mm, F.Cu at (29.7, 71.4)
- added U2: STM8S003F3U, MyOwn:UQFN-16_3x3mm_Pitch0.5mm, F.Cu at (29.7, 60.8)
- added U2: STM8S003F3U, MyOwn:UQFN-16_3x3mm_Pitch0.5mm, F.Cu at (29.7, 50.1)
- added U2: STM8S003F3U, MyOwn:UQFN-16_3x3mm_Pitch0.5mm, F.Cu at (29.7, 39.4)
- added U2: STM8S003F3U, MyOwn:UQFN-16_3x3mm_Pitch0.5mm, F.Cu at (29.7, 28.8)
- added U2: STM8S003F3U, MyOwn:UQFN-16_3x3mm_Pitch0.5mm, F.Cu at (29.7, 18.1)
- added U2: STM8S003F3U, MyOwn:UQFN-16_3x3mm_Pitch0.5mm, F.Cu at (63.2, 92.8)
- added U2: STM8S003F3U, MyOwn:UQFN-16_3x3mm_Pitch0.5mm, F.Cu at (63.2, 82.1)
- added U2: STM8S003F3U, MyOwn:UQFN-16_3x3mm_Pitch0.5mm, F.Cu at (63.2, 71.4)
- added U2: STM8S003F3U, MyOwn:UQFN-16_3x3mm_Pitch0.5mm, F.Cu at (63.2, 60.8)
- added U2: STM8S003F3U, MyOwn:UQFN-16_3x3mm_Pitch0.5mm, F.Cu at (63.2, 50.1)
- added U2: STM8S003F3U, MyOwn:UQFN-16_3x3mm_Pitch0.5mm, F.Cu at (63.2, 39.4)
- added U2: STM8S003F3U, MyOwn:UQFN-16_3x3mm_Pitch0.5mm, F.Cu at (63.2, 28.8)
- added U2: STM8S003F3U, MyOwn:UQFN-16_3x3mm_Pitch0.5mm, F.Cu at (63.2, 18.1)
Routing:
- net +3V3: track 0.00 -> 961.3 mm, vias 0 -> 36
- net VCC: track 767.7 -> 107.0 mm, vias 16 -> 0
- net PC7: track 84.3 -> 533.4 mm, vias 0 -> 36
- net GND: track 1592.9 -> 1184.8 mm, vias 48 -> 36
- net PC6: track 104.1 -> 416.9 mm, vias 16 -> 18
- net PC5: track 134.3 -> 444.1 mm, vias 0 -> 18
- net Net-(C2-Pad1): track 90.8 -> 363.7 mm, vias 0 -> 36
- net Net-(D1-Pad1): track 306.9 -> 36.2 mm
- net PD6/RX: track 315.2 -> 57.1 mm
- net PD4: track 392.2 -> 138.0 mm, vias 32 -> 0
- net PB5: track 515.4 -> 291.6 mm, vias 16 -> 18
- net PD5/TX: track 275.2 -> 102.7 mm, vias 0 -> 18
- net PB4: track 225.1 -> 380.5 mm, vias 0 -> 18
- net PC3: track 194.9 -> 39.8 mm
- net PD2: track 79.6 -> 219.2 mm, vias 0 -> 18
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- removed copper zone on B.Cu, net GND
- removed copper zone on F.Cu, net GND
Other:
- board size 95.5 x 95.5 mm -> 77.1 x 96 mm
- net class +12V removed
- net class Default: trace_width 0.3048 -> 0.1524; via_dia 0.8128 -> 0.635; via_drill 0.508 -> 0.3
- net class VCC removed
- rule pad_to_mask_clearance: 0.2 -> 0
- rule via_min_drill: 0.3048 -> 0.3
- rule via_min_size: 0.6096 -> 0.635
- board text added: "25 JUN 2017"
- board text added: "3V3"
- board text added: "G"
- board text added: "PC4"
- board text added: "PW"
- board text added: "RS"
- board text added: "RST"
- board text added: "S"
- board text added: "SW"
- board text added: "V-Cut line"
- board text removed: "+12V INPUT"
- board text removed: "C6"
- board text removed: "D1"
- board text removed: "NRST"
- board text removed: "PD4"
- board text removed: "PWR"
- board text removed: "RX"
- board text removed: "Rev1.0 Dec-2015 Designed by HW Wong"
- board text removed: "SWIM"
- board text removed: "TX"
- board text removed: "V-Cut"
